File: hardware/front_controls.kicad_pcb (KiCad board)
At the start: 2 copper layers, 99.8 x 99.8 mm, 87 parts, among them J1 Conn_01x02, J2 Conn_01x02, J3 Conn_01x02, J4 Conn_01x02, J5 Conn_01x02, J6 Conn_01x02, J7 Conn_01x02, J8 Conn_01x02, J9 Conn_01x02, P2 CONN_01X10, Q1 Q_PNP_BEC, U1 Adafruit_Metro_Mini, U10 G3VM-31BR, U2 G3VM-31BR, U3 G3VM-31BR, U4 G3VM-31BR, U5 G3VM-31BR, U6 G3VM-31BR, U7 G3VM-31BR, U8 G3VM-31BR, U9 G3VM-31BR

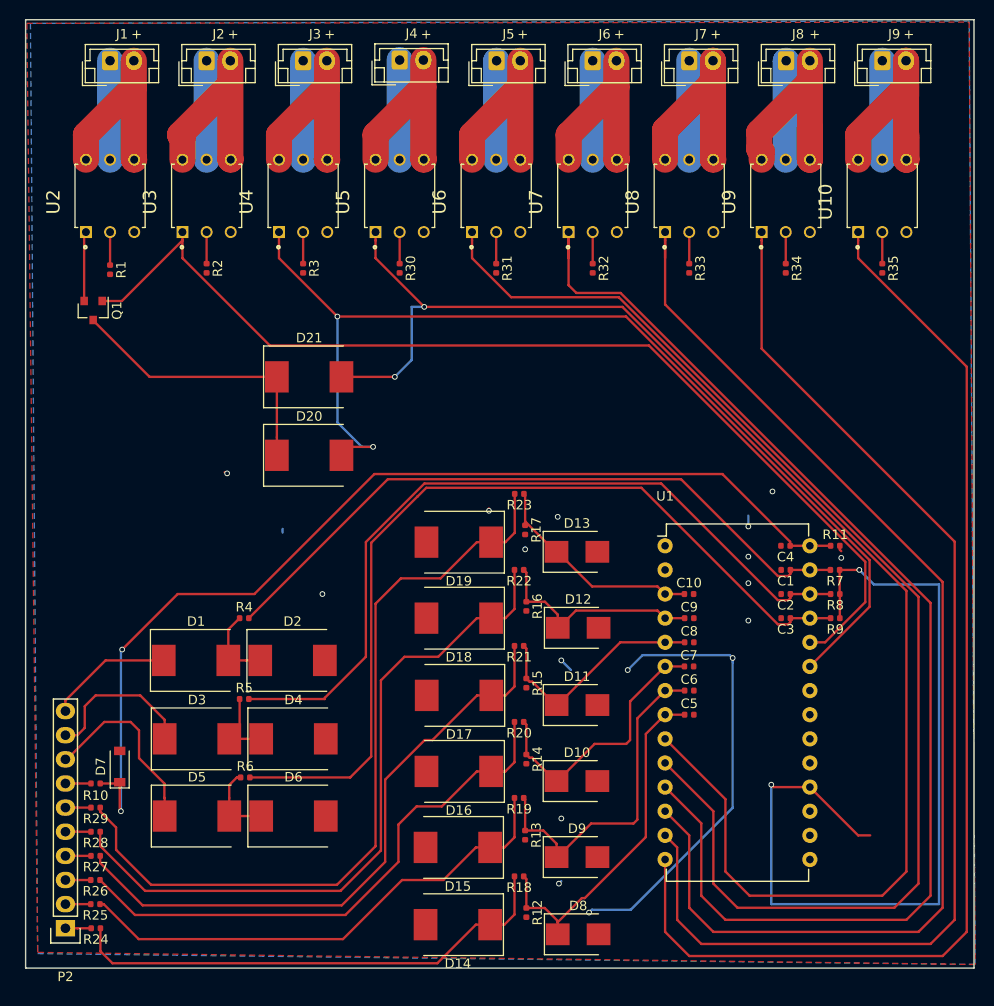
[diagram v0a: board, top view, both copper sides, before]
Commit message: Version 2 hardware files
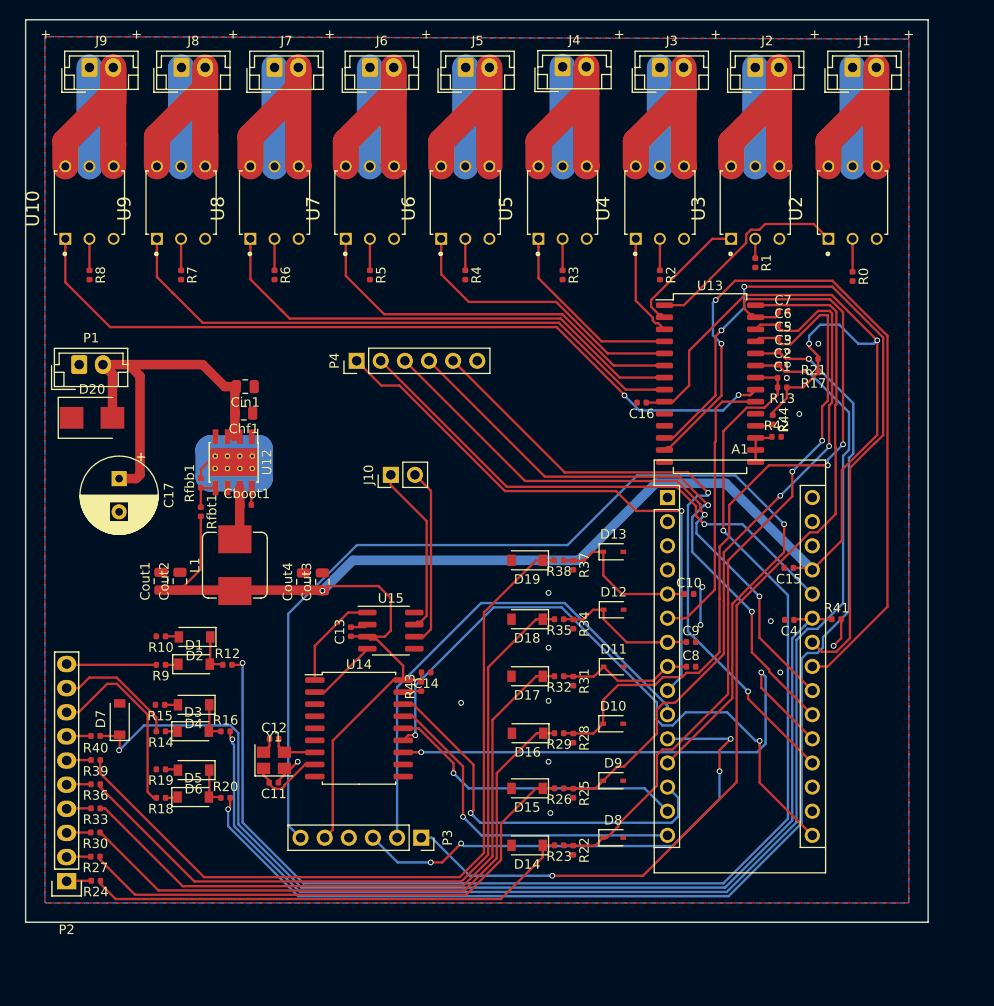
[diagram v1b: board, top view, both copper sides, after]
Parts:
- removed D21: D_Schottky, Diode_SMD:D_SMC
- removed Q1: Q_PNP_BEC, Package_TO_SOT_SMD:SOT-23
- removed the R16 at (139.1, 109.2)
- removed the R25 at (93.7, 140.6)
- removed the R26 at (93.7, 138.0)
- removed the R28 at (93.7, 133.0)
- removed the R29 at (93.7, 130.4)
- removed the R31 at (135.9, 73.7)
- removed the R32 at (146.1, 73.7)
- removed the R35 at (176.5, 73.7)
- removed U1: Adafruit_Metro_Mini, Adafruit:DIP-28_W15.24mm
- added A1: Arduino_Nano_v3.x, NANO:Arduino_Nano, F.Cu at (153.9, 97.8)
- added C11: 33pf, Capacitor_SMD:C_0402_1005Metric, F.Cu at (112.5, 127.8)
- added C12: 33pf, Capacitor_SMD:C_0402_1005Metric, F.Cu at (112.5, 123.2)
- added C13: 100nf, Capacitor_SMD:C_0402_1005Metric, F.Cu at (120.6, 111.9)
- added C14: 100nf, Capacitor_SMD:C_0402_1005Metric, F.Cu at (128.5, 116.2)
- added C15: 100nf, Capacitor_SMD:C_0402_1005Metric, F.Cu at (166.7, 105.2)
- added C16: 100nf, Capacitor_SMD:C_0402_1005Metric, F.Cu at (151.2, 87.8)
- added C17: 330uf, Capacitor_THT:CP_Radial_D8.0mm_P3.50mm, F.Cu at (96.2, 95.8)
- added Cboot1: 0.1uf, Capacitor_SMD:C_0402_1005Metric, F.Cu at (109.6, 98.6)
- added Chf1: 220nf, Capacitor_SMD:C_0805_2012Metric, F.Cu at (109.3, 88.9)
- added Cin1: 10uf, Capacitor_SMD:C_0805_2012Metric, F.Cu at (109.5, 86.1)
- added Cout1: 22uF, Capacitor_SMD:C_0805_2012Metric, F.Cu at (100.6, 106.6)
- added Cout2: 22uF, Capacitor_SMD:C_0805_2012Metric, F.Cu at (102.6, 106.6)
- added Cout3: 22uF, Capacitor_SMD:C_0805_2012Metric, F.Cu at (117.6, 106.7)
- added Cout4: 22uF, Capacitor_SMD:C_0805_2012Metric, F.Cu at (115.6, 106.7)
- added J10: Conn_01x02, Connector_PinHeader_2.54mm:PinHeader_1x02_P2.54mm_Vertical, F.Cu at (124.8, 95.4)
- added L1: 8uH, 14m, Inductor_SMD:L_Bourns_SRP7028A_7.3x6.6mm, F.Cu at (108.4, 104.9)
- added P1: PWR, Connector_JST:JST_EH_B2B-EH-A_1x02_P2.50mm_Vertical, F.Cu at (92.0, 83.8)
- added P3: HM-10, Connector_PinSocket_2.54mm:PinSocket_1x06_P2.54mm_Vertical, F.Cu at (128.0, 133.6)
- added P4: Conn_01x06, Connector_PinHeader_2.54mm:PinHeader_1x06_P2.54mm_Vertical, F.Cu at (121.2, 83.4)
- added R0: 500R, Resistor_SMD:R_0402_1005Metric, F.Cu at (173.4, 74.5)
- added R14: 1k, Resistor_SMD:R_0402_1005Metric, F.Cu at (100.6, 122.4)
- added R15: 1k, Resistor_SMD:R_0402_1005Metric, F.Cu at (100.5, 119.6)
- added R17: 100k, Resistor_SMD:R_0402_1005Metric, F.Cu at (169.3, 84.6)
- added R18: 1k, Resistor_SMD:R_0402_1005Metric, F.Cu at (100.6, 129.4)
- added R19: 1k, Resistor_SMD:R_0402_1005Metric, F.Cu at (100.6, 126.4)
- added R20: 1k, Resistor_SMD:R_0402_1005Metric, F.Cu at (107.4, 129.4)
- added R36: 10R, Resistor_SMD:R_0402_1005Metric, F.Cu at (93.7, 128.0)
- added R39: 10R, Resistor_SMD:R_0402_1005Metric, F.Cu at (93.7, 125.4)
- added R4: 500R, Resistor_SMD:R_0402_1005Metric, F.Cu at (132.6, 74.4)
- added R40: 10R, Resistor_SMD:R_0402_1005Metric, F.Cu at (93.7, 122.9)
- added R42: 4K7 1%, Resistor_SMD:R_0402_1005Metric, F.Cu at (165.4, 91.4)
- added R43: 100k, Resistor_SMD:R_0402_1005Metric, F.Cu at (128.0, 117.7)
- added R44: 100k, Resistor_SMD:R_0402_1005Metric, F.Cu at (165.0, 89.6)
- added R5: 500R, Resistor_SMD:R_0402_1005Metric, F.Cu at (122.6, 74.4)
- added R7: 500R, Resistor_SMD:R_0402_1005Metric, F.Cu at (102.7, 74.4)
- added R9: 1k, Resistor_SMD:R_0402_1005Metric, F.Cu at (100.6, 115.4)
- added Rfbb1: 24K9 1%, Resistor_SMD:R_0402_1005Metric, F.Cu at (104.8, 96.3)
- added Rfbt1: 100k 1%, Resistor_SMD:R_0402_1005Metric, F.Cu at (104.8, 99.3)
- added U12: LMR33630ADDA, NANO:Texas_HSOP-8-1EP_3.9x4.9mm_P1.27mm_ThermalVias, F.Cu at (108.3, 94.1)
- added U13: MCP23017-E/SO, Package_SO:SOIC-28W_7.5x18.7mm_P1.27mm, F.Cu at (158.4, 85.8)
- added U14: MCP2515-xSO, Package_SO:SOIC-18W_7.5x11.6mm_P1.27mm, F.Cu at (121.5, 122.1)
- added U15: TJA1051T, Package_SO:SOIC-8_3.9x4.9mm_P1.27mm, F.Cu at (124.8, 111.8)
- added Y1: 12Mhz, Crystal:Crystal_SMD_3225-4Pin_3.2x2.5mm, F.Cu at (112.5, 125.5)
- D1, D14, D15, D16, D17, D18, D19, D2, D3, D4, D5, D6: footprint Diode_SMD:D_SMC -> Diode_SMD:D_SOD-123
- D10, D11, D12, D13, D8, D9: value 4.7 -> 4.7V Zener; footprint Diode_SMD:D_SMB -> Diode_SMD:D_SOD-323
- D20: value D_Schottky -> 15V standoff; footprint Diode_SMD:D_SMC -> Diode_SMD:D_SMB
- D7: value 5.1 -> 5.1V Zener
- R1, R2, R3: value 500 -> 500R
- R10: value 10 -> 1k
- R24, R27: value 10 -> 10R
- R30, R33: value 500 -> 10R
- R34: value 500 -> 100k
- R6: value 1k -> 500R
- R8: value 100k -> 500R
- moved R8 85.4 mm to (93.1, 74.4), turned to 270 degrees
- moved R33 84.5 mm to (93.7, 130.5), turned to 180 degrees
- moved J9 83.5 mm to (93.1, 52.5)
- moved U10 83.5 mm to (93.1, 66.7)
- moved J1 78.2 mm to (173.4, 52.5)
- moved U2 78.2 mm to (173.4, 66.7)
- moved R1 67.9 mm to (163.2, 73.1)
- moved R30 67.5 mm to (93.7, 133.0), turned to 180 degrees
- moved U9 63.7 mm to (102.7, 66.7)
- moved J8 63.7 mm to (102.8, 52.5)
- moved J2 57.8 mm to (163.2, 52.5)
- moved U3 57.8 mm to (163.2, 66.7)
- moved R6 53.0 mm to (112.6, 74.4), turned to 270 degrees
- moved R2 47.7 mm to (153.1, 74.4)
- moved J7 43.7 mm to (112.6, 52.5)
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- renumbered R4 to R12, R7 to R13, R5 to R16, R9 to R21, R12 to R22, R18 to R23, R13 to R25, R19 to R26, R14 to R28, R20 to R29, R15 to R31, R21 to R32, R22 to R35, R17 to R37, R23 to R38, R11 to R41
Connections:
- net Net-(C1-Pad1) renamed /IN_LOW1
- net Net-(C10-Pad1) renamed /IN_HIGH6
- net Net-(C5-Pad1) renamed /IN_HIGH1
- net Net-(C6-Pad1) renamed /IN_HIGH2
- net Net-(C7-Pad1) renamed /IN_HIGH3
- net Net-(C8-Pad1) renamed /IN_HIGH4
- C2 pad 1: Net-(C2-Pad1) -> /IN_LOW2
- C3 pad 1: Net-(C3-Pad1) -> /IN_LOW3
- C4 pad 1: Net-(C4-Pad1) -> /IN_AN1
- C9 pad 1: Net-(C9-Pad1) -> /IN_HIGH5
- D12 pad 1: Net-(C9-Pad1) -> /IN_HIGH5
- D2 pad 2: GND -> Net-(D2-Pad2)
- D20 pad 1: Net-(D20-Pad1) -> GND
- D20 pad 2: Net-(D20-Pad2) -> Net-(C17-Pad1)
- D4 pad 2: GND -> Net-(D4-Pad2)
- D6 pad 2: GND -> Net-(D6-Pad2)
- D7 pad 1: Net-(C4-Pad1) -> /IN_AN1
- P2 pad 10: Net-(D1-Pad1) -> Net-(P2-Pad10)
- P2 pad 8: Net-(D5-Pad1) -> Net-(P2-Pad8)
- P2 pad 9: Net-(D3-Pad1) -> Net-(P2-Pad9)
- R10 pad 1: Net-(P2-Pad7) -> Net-(D2-Pad2)
- R10 pad 2: Net-(C4-Pad1) -> GND
- R16 pad 2: Net-(C2-Pad1) -> /IN_LOW2
- R21 pad 2: Net-(C3-Pad1) -> /IN_LOW3
- R27 pad 1: Net-(D17-Pad1) -> Net-(D15-Pad1)
- R27 pad 2: Net-(P2-Pad4) -> Net-(P2-Pad2)
- R30 pad 1: Net-(R30-Pad1) -> Net-(D16-Pad1)
- R30 pad 2: GND -> Net-(P2-Pad3)
- R33 pad 1: Net-(R33-Pad1) -> Net-(D17-Pad1)
- R33 pad 2: GND -> Net-(P2-Pad4)
- R34 pad 1: Net-(R34-Pad1) -> /IN_HIGH5
- R35 pad 1: Net-(C9-Pad1) -> /IN_HIGH5
- R41 pad 1: Net-(C4-Pad1) -> /IN_AN1
- R6 pad 1: Net-(D5-Pad2) -> Net-(R6-Pad1)
- R6 pad 2: Net-(C3-Pad1) -> GND
- R8 pad 1: VCC -> Net-(R8-Pad1)
- R8 pad 2: Net-(C2-Pad1) -> GND
- U10 pad 1: Net-(U1-Pad13) -> /OUT_U10
- U10 pad 2: Net-(R35-Pad1) -> Net-(R8-Pad1)
- U10 pad 4: Net-(U10-Pad4) -> (no net)
- U2 pad 1: Net-(Q1-Pad2) -> /OUT_U2
- U2 pad 2: Net-(R1-Pad1) -> Net-(R0-Pad1)
- U2 pad 4: Net-(U2-Pad4) -> (no net)
- U3 pad 1: Net-(Q1-Pad1) -> /OUT_U3
- U3 pad 2: Net-(R2-Pad1) -> Net-(R1-Pad1)
- U3 pad 4: Net-(U3-Pad4) -> (no net)
- U4 pad 1: Net-(D20-Pad2) -> /OUT_U4
- U4 pad 2: Net-(R3-Pad1) -> Net-(R2-Pad1)
- U4 pad 4: Net-(U4-Pad4) -> (no net)
- U5 pad 1: Net-(D21-Pad2) -> /OUT_U5
- U5 pad 2: Net-(R30-Pad1) -> Net-(R3-Pad1)
- U5 pad 4: Net-(U5-Pad4) -> (no net)
- U6 pad 1: Net-(U1-Pad9) -> /OUT_U6
- U6 pad 4: Net-(U6-Pad4) -> (no net)
- U7 pad 1: Net-(U1-Pad10) -> /OUT_U7
- U8 pad 1: Net-(U1-Pad11) -> /OUT_U8
- U8 pad 2: Net-(R33-Pad1) -> Net-(R6-Pad1)
- U9 pad 1: Net-(U1-Pad12) -> /OUT_U9
- U9 pad 2: Net-(R34-Pad1) -> Net-(R7-Pad1)
- U9 pad 4: Net-(U9-Pad4) -> (no net)
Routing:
- net Net-(D21-Pad2): track 155.5 -> 0.00 mm, vias 2 -> 0
- net /IN_LOW2: track 0.00 -> 133.4 mm, vias 0 -> 2
- net Net-(U1-Pad9): track 133.2 -> 0.00 mm
- net Net-(U1-Pad10): track 130.3 -> 0.00 mm
- net /IN_LOW3: track 0.00 -> 129.4 mm, vias 0 -> 2
- net Net-(U1-Pad11): track 125.9 -> 0.00 mm
- net Net-(U1-Pad12): track 121.5 -> 0.00 mm
- net VCC: track 92.7 -> 214.1 mm, vias 2 -> 3
- net Net-(U1-Pad13): track 119.9 -> 0.00 mm
- net /IN_AN1: track 0.00 -> 117.5 mm, vias 0 -> 1
- net /BT_EN: track 0.00 -> 114.7 mm, vias 0 -> 1
- net Net-(D20-Pad2): track 111.5 -> 0.00 mm, vias 2 -> 0
- net Net-(Q1-Pad1): track 110.8 -> 0.00 mm
- net Net-(C4-Pad1): track 107.9 -> 0.00 mm, vias 2 -> 0
- net /BT_STATE: track 0.00 -> 102.1 mm, vias 0 -> 1
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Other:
- board size 99.8 x 99.8 mm -> 95 x 95 mm
- board text added: "EDL front_controls V. 0.2.0"
- board text removed: "EDL front_controls V. 0.1.0"
